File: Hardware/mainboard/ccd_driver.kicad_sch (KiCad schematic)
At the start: 61 parts, among them Q801 BC847BPN, U801 74HC4053, U802 74HC2G17, U803 74HC2G17, U804 74HC2G17, U805 74HC2G17, U806 74HC2G17, U807 74HC2G17, U808 CD4053B, U809 UCC27517A, U810 UCC27517A, U811 UCC27517A, U812 UCC27517A

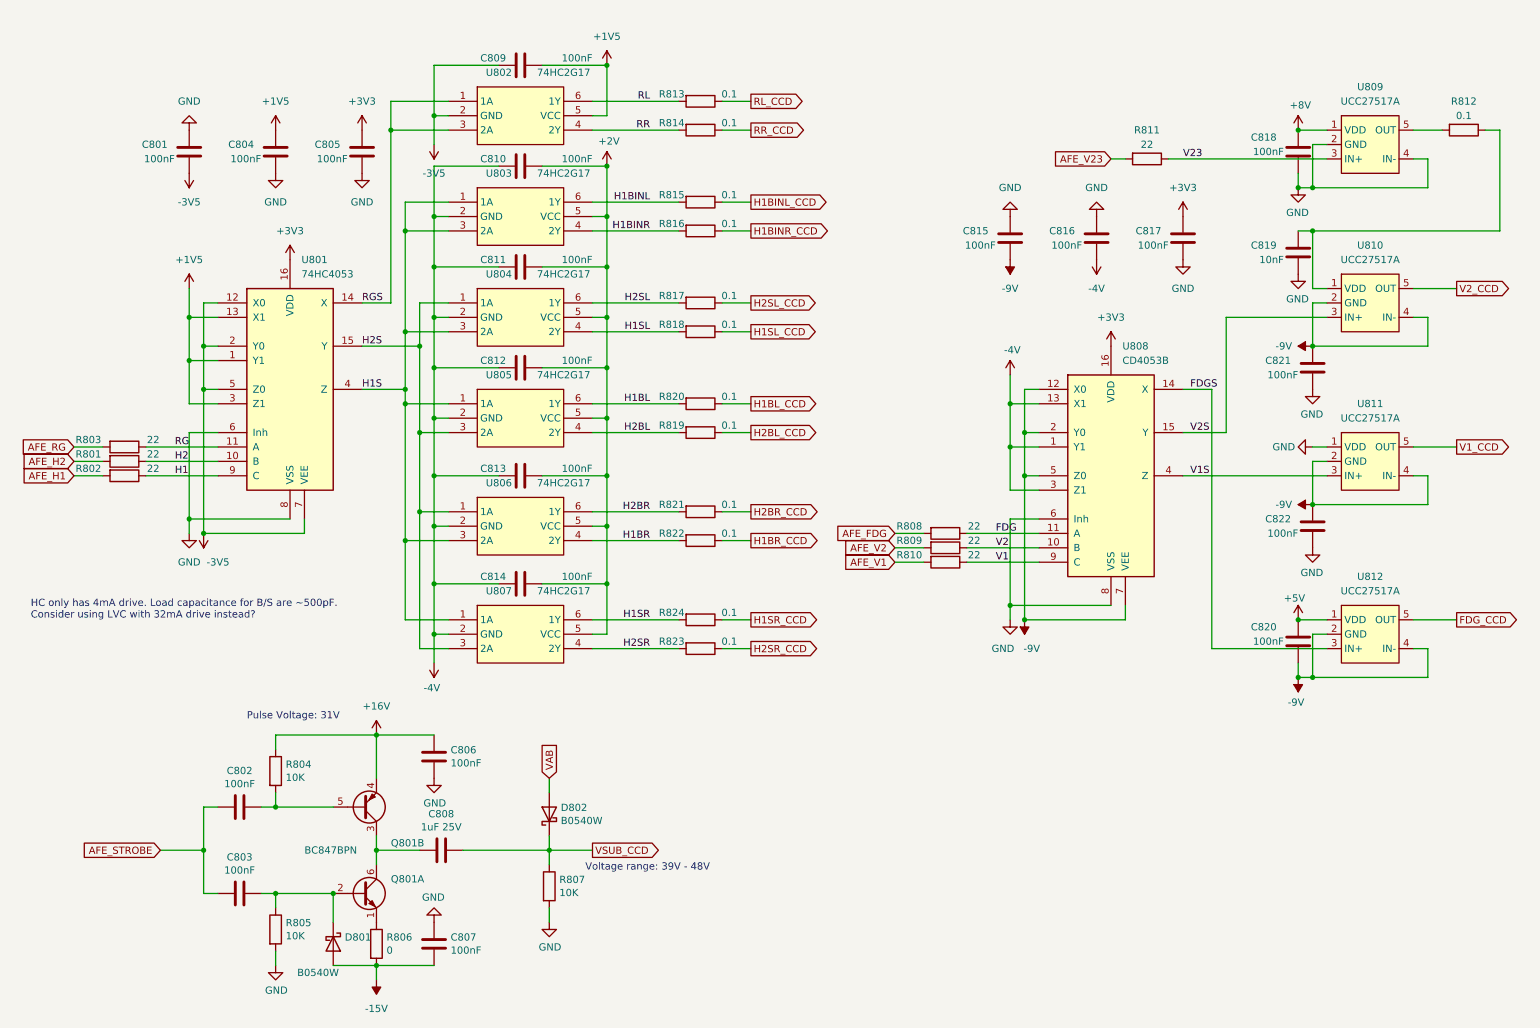
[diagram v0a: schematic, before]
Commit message: Working towards pcb r0.7
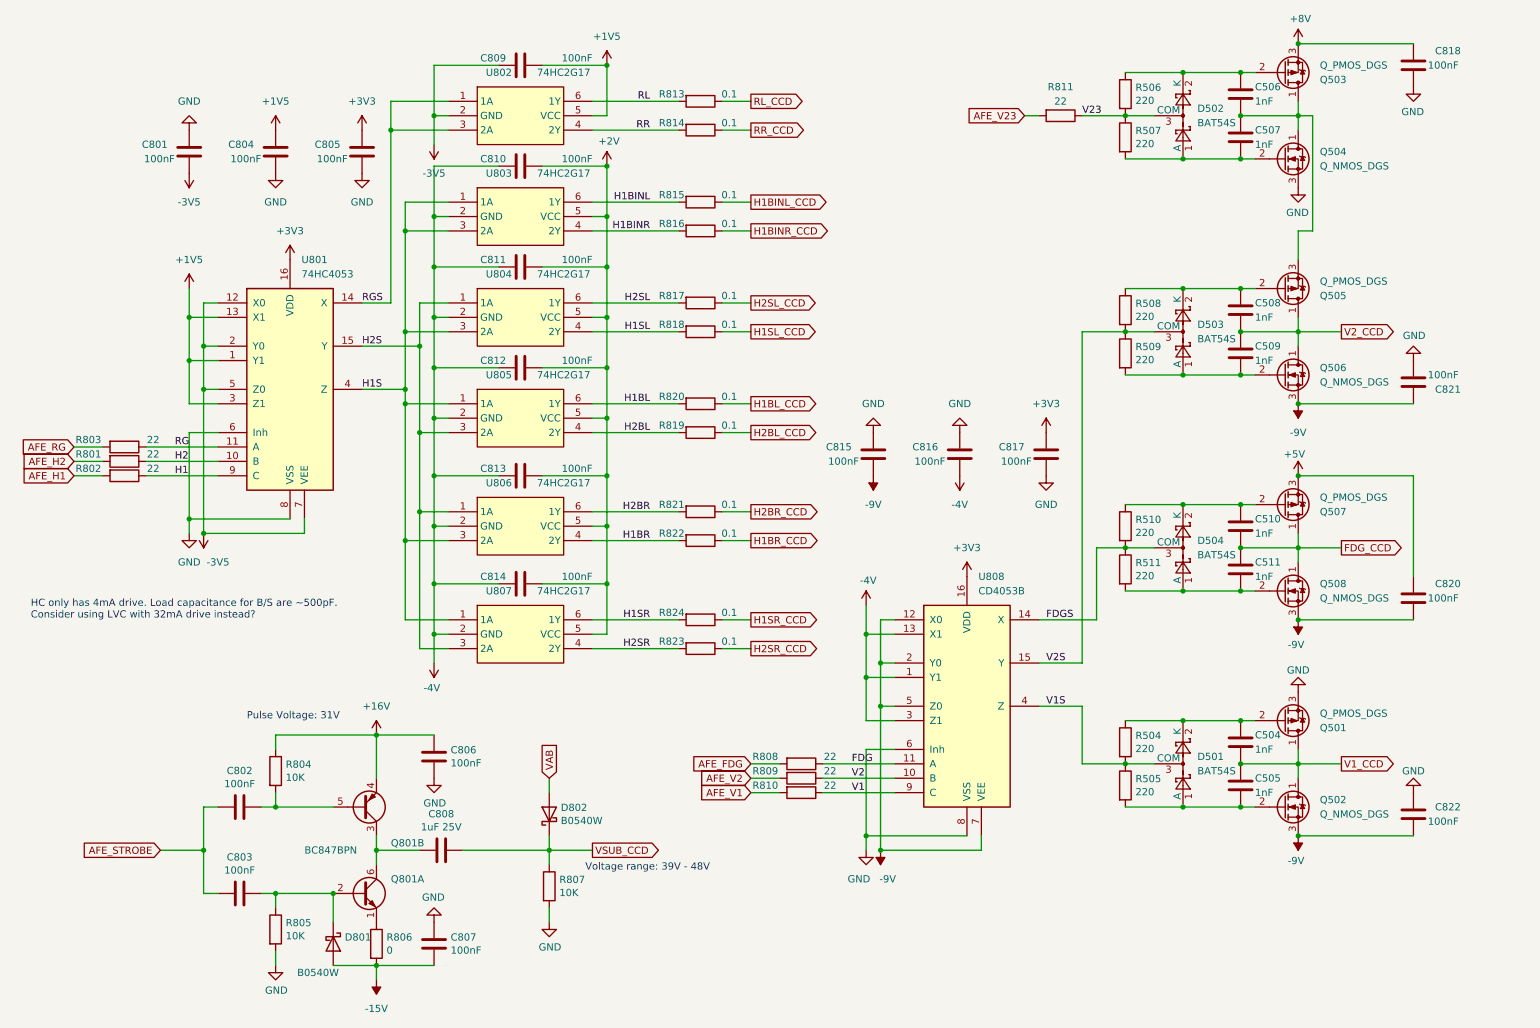
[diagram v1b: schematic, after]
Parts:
- removed C819: 10nF, Capacitor_SMD:C_0402_1005Metric, symbol Device:C
- removed R812: 0.1, Resistor_SMD:R_0603_1608Metric, symbol Device:R
- removed U809, U810, U811, U812: UCC27517A, Package_TO_SOT_SMD:SOT-23-5, symbol Sitina:UCC27517A
- added C504, C505, C506, C507, C508, C509, C510, C511: 1nF, Capacitor_SMD:C_0402_1005Metric, symbol Device:C
- added D501, D502, D503, D504: BAT54S, Package_TO_SOT_SMD:SOT-23, symbol Diode:BAT54S
- added Q501, Q503, Q505, Q507: Q_PMOS_DGS, symbol Device:Q_PMOS_DGS
- added Q502, Q504, Q506, Q508: Q_NMOS_DGS, symbol Device:Q_NMOS_DGS
- added R504, R505, R506, R507, R508, R509, R510, R511: 220, Resistor_SMD:R_0402_1005Metric, symbol Device:R
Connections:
- net +5V: now also Q507.3 (S)
- net +8V: now also Q503.3 (S)
- net -9V: now also C822.1, Q502.3 (S), Q506.3 (S), Q508.3 (S); no longer C822.2
- net FDGS: now also D504.3 (COM), R510.2, R511.1
- net FDG_CCD: now also C510.1, C511.2, Q507.1 (D), Q508.1 (D)
- net GND: now also C822.2, Q501.3 (S), Q504.3 (S); no longer C822.1
- net V1S: now also D501.3 (COM), R504.2, R505.1
- net V1_CCD: now also C504.1, C505.2, Q501.1 (D), Q502.1 (D)
- net V23: now also D502.3 (COM), R506.2, R507.1
- net V2S: now also D503.3 (COM), R508.2, R509.1
- net V2_CCD: now also C508.1, C509.2, Q505.1 (D), Q506.1 (D)
- new net: C510.2, D504.2 (K), Q507.2 (G), R510.1
- new net: C508.2, D503.2 (K), Q505.2 (G), R508.1
- new net: C511.1, D504.1 (A), Q508.2 (G), R511.2
- new net: C509.1, D503.1 (A), Q506.2 (G), R509.2
- new net: C505.1, D501.1 (A), Q502.2 (G), R505.2
- new net: C507.1, D502.1 (A), Q504.2 (G), R507.2
- new net: C506.2, D502.2 (K), Q503.2 (G), R506.1
- new net: C504.2, D501.2 (K), Q501.2 (G), R504.1
- new net: C506.1, C507.2, Q503.1 (D), Q504.1 (D), Q505.3 (S)
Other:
- moved on the sheet: C815, C816, C817, C818, C820, C821, C822, R808, R809, R810, R811, U808
